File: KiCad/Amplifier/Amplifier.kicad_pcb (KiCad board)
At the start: 4 copper layers, 165.9 x 144.3 mm, 152 parts, among them J1 Input, J2 Enable, J3 Vp_8V, J4 Vn_-5V, J5 Output, J6 Input_56V, Q1 BD139, Q10 BD140, Q2 IXTH90P10P, Q4 BD139, Q5A1 BSC340N08NS3G, Q6 BD139, Q7 BD139, Q8 BD139, Q9 BD140, U1 AD8017ARZ, U2 AD8021AR, U3 BLF188XRU, U4 AD8033, U5 LT3014xS5

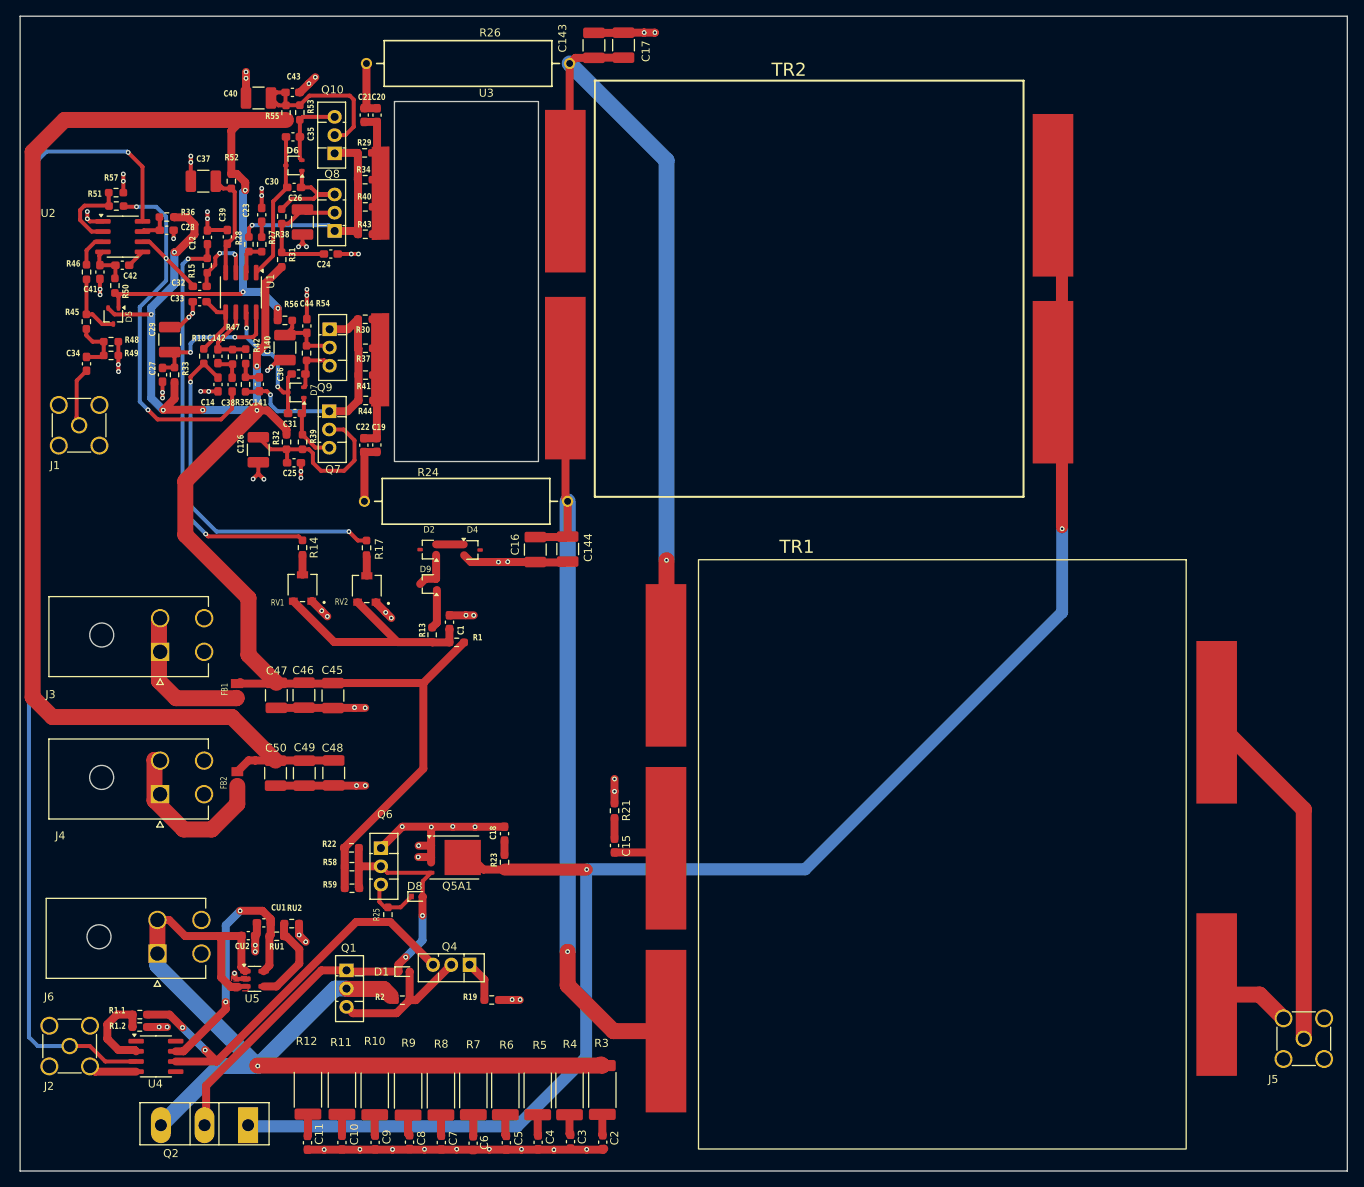
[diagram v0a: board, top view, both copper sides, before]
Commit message: Update PCB
update PCB
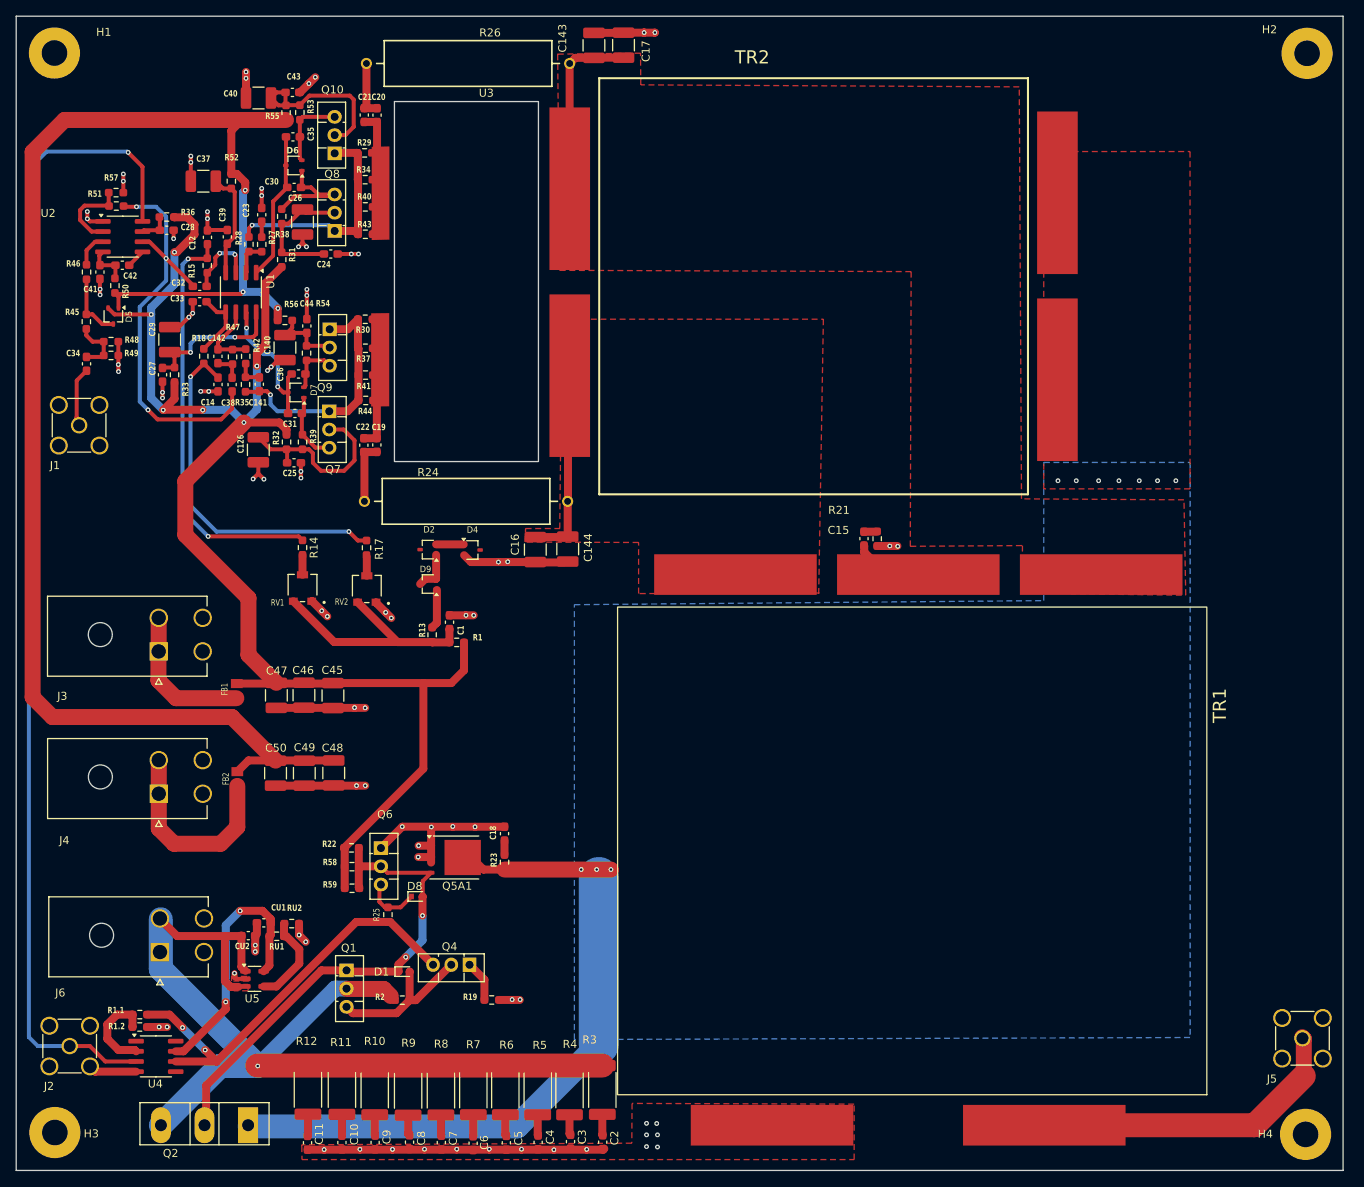
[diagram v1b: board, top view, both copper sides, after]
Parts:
- added H1: MountingHole, MountingHole:MountingHole_3.2mm_M3_Pad, F.Cu at (34.6, 21.7)
- added H2: MountingHole, MountingHole:MountingHole_3.2mm_M3_Pad, F.Cu at (191.2, 21.8)
- added H3: MountingHole, MountingHole:MountingHole_3.2mm_M3_Pad, F.Cu at (34.6, 156.7)
- added H4: MountingHole, MountingHole:MountingHole_3.2mm_M3_Pad, F.Cu at (191.0, 156.9)
- moved C15 49.4 mm to (135.8, 82.4)
- moved R21 47.3 mm to (137.4, 82.4), turned to -90 degrees
- moved TR2 27.7 mm to (129.7, 56.2)
- moved TR1 2.88 mm to (142.1, 118.9), turned to 180 degrees
- moved J6 0.37 mm to (47.8, 134.1)
- moved J3 0.19 mm to (47.6, 96.5)
- moved J5 0.17 mm to (190.6, 144.9)
- moved J4 0.17 mm to (47.6, 114.3)
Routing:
- net Output_56V: track 209.9 -> 88.3 mm, vias 2 -> 10
- net /HF Part/D1: track 103.7 -> 23.4 mm, vias 1 -> 0
- net /HF Part/D2: track 99.3 -> 23.7 mm, vias 1 -> 0
- net GND: track 198.2 -> 188.1 mm, vias 77 -> 83
- net Net-(J4-Pin_1): track 20.5 -> 25.2 mm
- net /HF Part/Output: track 44.1 -> 39.9 mm
- net Vp: track 177.7 -> 180.0 mm
- net Net-(TR1-PM): track 6.70 -> 8.81 mm
- net Input_56V: track 128.7 -> 127.4 mm
- net Net-(C15-Pad1): track 2.58 -> 1.67 mm
- added copper zone on F.Cu, net /HF Part/D1
- added copper zone on F.Cu, net /HF Part/D2
- added copper zone on B.Cu, net Output_56V
- added copper zone on F.Cu, net Output_56V
